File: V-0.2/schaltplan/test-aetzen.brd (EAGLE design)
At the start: 78.6 x 50.8 mm, 53 parts, among them IC1 MEGA32-A, IC2 NE5532N, Q1 BUZ21, X1 BU-SMB-H, X2 PN61729-S

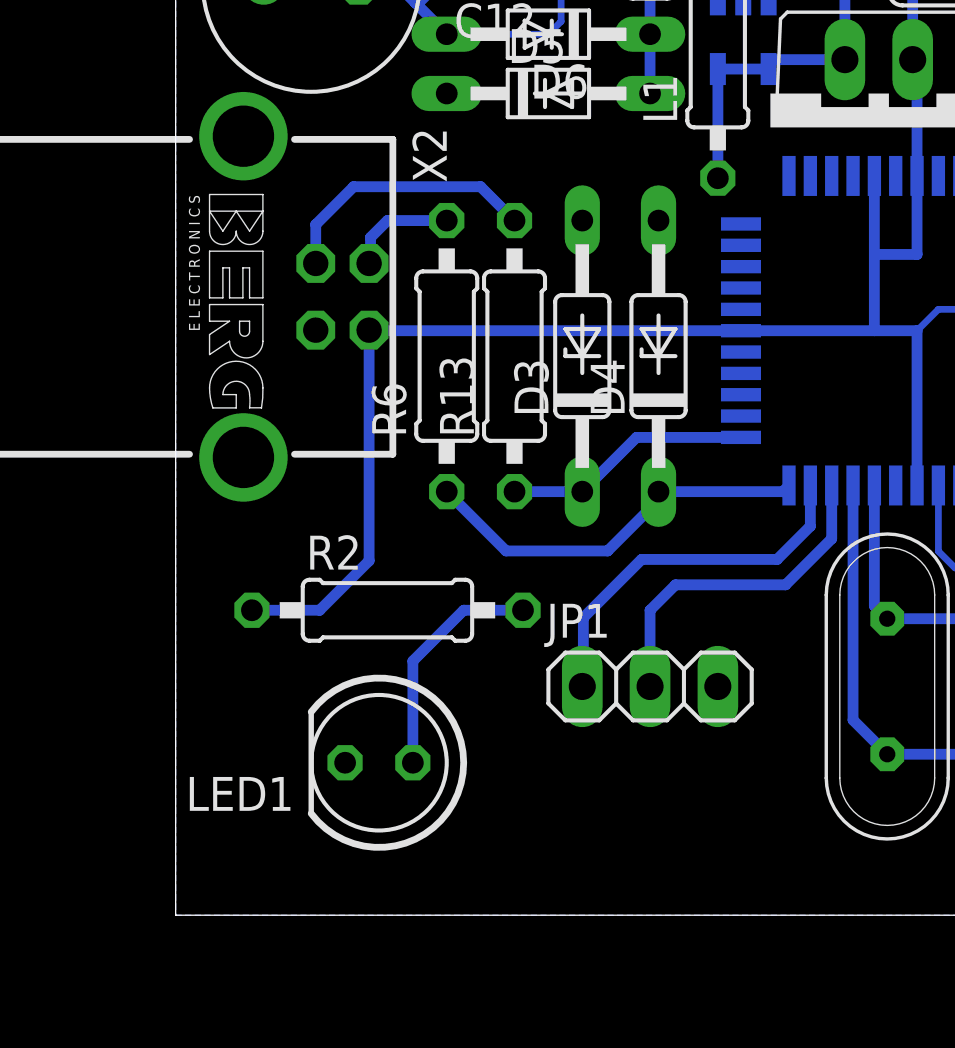
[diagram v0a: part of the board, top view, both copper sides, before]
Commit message: i have no flash drive with me :(
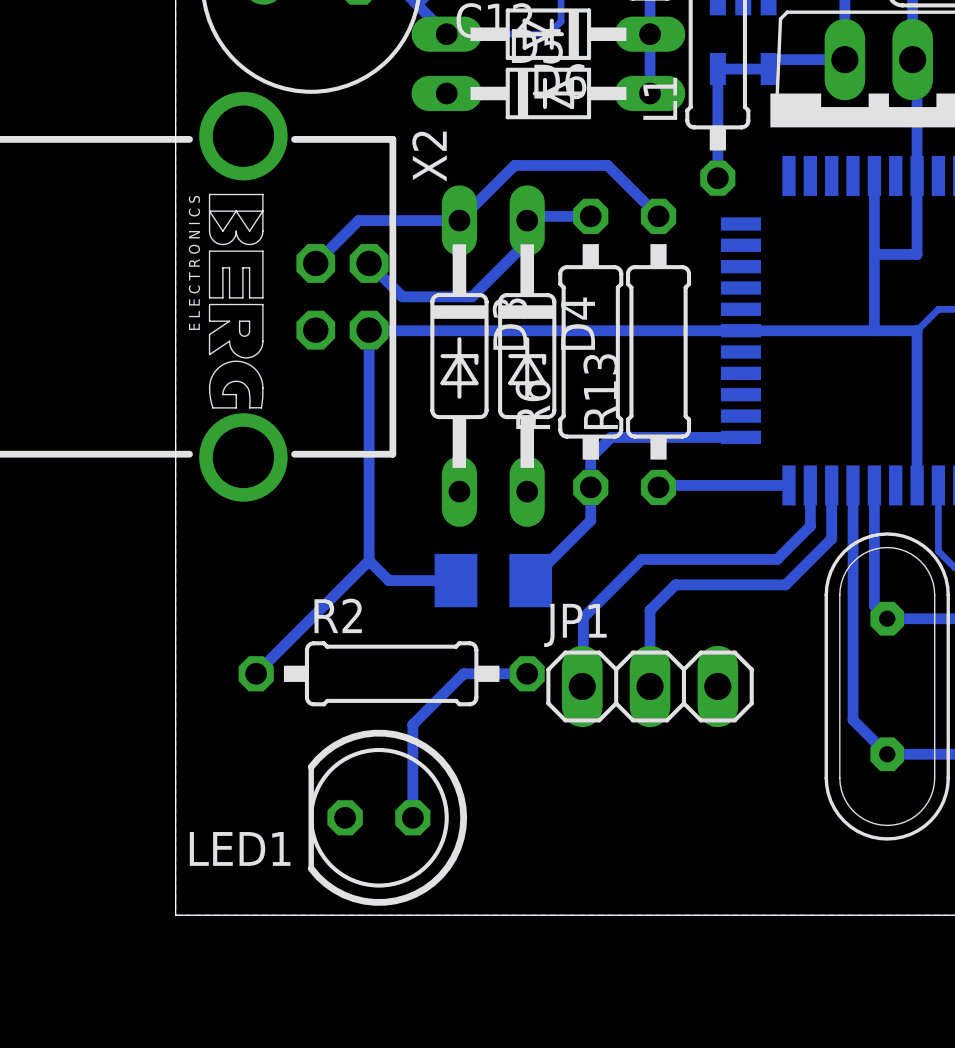
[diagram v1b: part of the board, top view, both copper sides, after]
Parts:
- added R17: 10k, rcl:M1206
- moved R13 5.40 mm to (18.1, 21.1)
- moved R6 5.40 mm to (15.6, 21.1)
- moved D4 4.92 mm to (13.2, 21.0), turned to 270 degrees
- moved D3 4.60 mm to (10.6, 21.0), turned to 270 degrees
- moved R2 2.39 mm to (8.10, 9.05)
- moved LED1 2.06 mm to (7.62, 3.65)
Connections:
- net N$13: now also D4.C
- net N$14: now also D3.C
- net N$2: now also IC1.12, R17.2; no longer D4.C, IC1.11
- net N$5: now also IC1.11; no longer D3.C, IC1.12
- net VCC: now also R17.1
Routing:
- net N$13: track 4.11 -> 10.5 mm
- net N$14: track 10.0 -> 15.2 mm
- net N$5: track 9.33 -> 4.92 mm
- net VCC: track 124.4 -> 128.8 mm
- net N$2: track 15.0 -> 11.5 mm
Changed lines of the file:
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@@
 <layer number="22" name="bPlace" color="7" fill="1" visible="no" active="yes"/>
 <layer number="23" name="tOrigins" color="15" fill="1" visible="yes" active="yes"/>
-<layer number="24" name="bOrigins" color="15" fill="1" visible="no" active="yes"/>
+<layer number="24" name="bOrigins" color="15" fill="1" visible="yes" active="yes"/>
 <layer number="25" name="tNames" color="7" fill="1" visible="yes" active="yes"/>
 <layer number="26" name="bNames" color="7" fill="1" visible="no" active="yes"/>
@@
 <element name="D1" library="diode" package="DO35-7" value="1N4148DO35-7" x="44.45" y="37.465"/>
 <element name="D2" library="diode" package="DO35-7" value="1N4148DO35-7" x="44.45" y="35.2425" rot="R180"/>
-<element name="D3" library="diode" package="DO35Z10" value="" x="15.24" y="20.955" rot="R90"/>
-<element name="D4" library="diode" package="DO35Z10" value="" x="18.0975" y="20.955" rot="R90"/>
+<element name="D3" library="diode" package="DO35Z10" value="" x="10.63625" y="20.955" rot="R270"/>
+<element name="D4" library="diode" package="DO35Z10" value="" x="13.17625" y="20.955" rot="R270"/>
 <element name="D5" library="diode" package="DO34-7" value="BAT81" x="13.97" y="30.7975"/>
 <element name="D6" library="diode" package="DO34-7" value="BAT81" x="13.97" y="33.02" rot="R180"/>
@@
 <element name="JP2" library="jumper" package="JP4Q" value="" x="54.13375" y="27.78125" rot="R90"/>
 <element name="L1" library="rcl" package="0207/10" value="" x="20.32" y="32.7025" rot="R90"/>
-<element name="LED1" library="led" package="LED5MM" value="" x="7.62" y="5.715" rot="R180"/>
+<element name="LED1" library="led" package="LED5MM" value="" x="7.62" y="3.65125" rot="R180"/>
 <element name="Q1" library="transistor-fet" package="TO220V" value="BUZ21" x="27.6225" y="29.5275" rot="R180"/>
 <element name="QG1" library="crystal" package="SM77H" value="SM77H" x="43.18" y="15.24" rot="MR0">
@@
 <element name="R11" library="rcl" package="M1206" value="10k" x="63.02375" y="16.98625" rot="MR0"/>
 <element name="R12" library="rcl" package="M1206" value="10k" x="59.84875" y="9.2075" rot="MR270"/>
-<element name="R13" library="rcl" package="0207/10" value="33R" x="12.7" y="20.955" rot="R90"/>
-<element name="R2" library="rcl" package="0207/10" value="" x="7.9375" y="11.43"/>
+<element name="R13" library="rcl" package="0207/10" value="33R" x="18.0975" y="21.11375" rot="R90"/>
+<element name="R2" library="rcl" package="0207/10" value="" x="8.09625" y="9.04875"/>
 <element name="R3" library="rcl" package="RTRIM64Y" value="" x="70.32625" y="23.65375" rot="R270"/>
 <element name="R4" library="rcl" package="M1206" value="10k" x="34.925" y="6.0325" rot="MR270"/>
 <element name="R5" library="rcl" package="M1206" value="10k" x="34.6075" y="29.5275" rot="MR0"/>
-<element name="R6" library="rcl" package="0207/10" value="33R" x="10.16" y="20.955" rot="R90"/>
+<element name="R6" library="rcl" package="0207/10" value="33R" x="15.5575" y="21.11375" rot="R90"/>
 <element name="R7" library="rcl" package="0207/10" value="" x="17.145" y="40.64" rot="R180"/>
 <element name="R8" library="rcl" package="0207/10" value="" x="17.145" y="43.18"/>
@@
 <element name="JP1" library="pinhead" package="1X03" value="" x="17.78" y="8.5725"/>
 <element name="R16" library="rcl" package="M1206" value="10k" x="33.17875" y="37.30625" rot="MR270"/>
+<element name="R17" library="rcl" package="M1206" value="10k" x="11.90625" y="12.54125" rot="MR180"/>
 </elements>
 <signals>
@@
 <contactref element="R4" pad="2"/>
 <wire x1="7.25" y1="21.9275" x2="7.25" y2="13.2825" width="0.4064" layer="16"/>
-<wire x1="7.25" y1="13.2825" x2="5.3975" y2="11.43" width="0.4064" layer="16"/>
-<wire x1="5.3975" y1="11.43" x2="2.8575" y2="11.43" width="0.4064" layer="16"/>
+<wire x1="7.25" y1="13.2825" x2="3.01625" y2="9.04875" width="0.4064" layer="16"/>
 <wire x1="45.085" y1="5.08" x2="45.085" y2="3.175" width="0.4064" layer="16"/>
 <wire x1="45.085" y1="3.175" x2="44.1325" y2="2.2225" width="0.4064" layer="16"/>
@@
 <wire x1="28.41625" y1="37.30625" x2="27.6225" y2="36.5125" width="0.254" layer="16"/>
 <wire x1="27.6225" y1="36.5125" x2="27.6225" y2="35.2425" width="0.254" layer="16"/>
+<contactref element="R17" pad="1"/>
+<wire x1="10.50625" y1="12.54125" x2="7.99125" y2="12.54125" width="0.4064" layer="16"/>
+<wire x1="7.99125" y1="12.54125" x2="7.25" y2="13.2825" width="0.4064" layer="16"/>
 <wire x1="45.73" y1="13.34" x2="45.085" y2="5.08" width="0" layer="19" extent="16-16"/>
 </signal>
@@
 <contactref element="R2" pad="2"/>
 <contactref element="LED1" pad="A"/>
-<wire x1="13.0175" y1="11.43" x2="10.795" y2="11.43" width="0.4064" layer="16"/>
-<wire x1="10.795" y1="11.43" x2="8.89" y2="9.525" width="0.4064" layer="16"/>
-<wire x1="8.89" y1="9.525" x2="8.89" y2="5.715" width="0.4064" layer="16"/>
+<wire x1="13.17625" y1="9.04875" x2="10.795" y2="9.04875" width="0.4064" layer="16"/>
+<wire x1="10.795" y1="9.04875" x2="8.89" y2="7.14375" width="0.4064" layer="16"/>
+<wire x1="8.89" y1="7.14375" x2="8.89" y2="3.65125" width="0.4064" layer="16"/>
 </signal>
 <signal name="N$25">
@@
 </signal>
 <signal name="N$2">
+<contactref element="R6" pad="1"/>
+<contactref element="IC1" pad="12"/>
+<contactref element="R17" pad="2"/>
+<wire x1="21.1875" y1="17.9075" x2="16.32" y2="17.9075" width="0.4064" layer="16"/>
+<wire x1="16.32" y1="17.9075" x2="15.5575" y2="17.145" width="0.4064" layer="16"/>
+<wire x1="15.5575" y1="17.145" x2="15.5575" y2="16.03375" width="0.4064" layer="16"/>
+<wire x1="15.5575" y1="16.03375" x2="15.5575" y2="14.7925" width="0.4064" layer="16"/>
+<wire x1="15.5575" y1="14.7925" x2="13.30625" y2="12.54125" width="0.4064" layer="16"/>
+</signal>
+<signal name="N$5">
+<contactref element="R13" pad="1"/>
 <contactref element="IC1" pad="11"/>
-<contactref element="R6" pad="1"/>
-<contactref element="D4" pad="C"/>
-<wire x1="10.16" y1="15.875" x2="12.3825" y2="13.6525" width="0.4064" layer="16"/>
-<wire x1="12.3825" y1="13.6525" x2="16.1925" y2="13.6525" width="0.4064" layer="16"/>
-<wire x1="16.1925" y1="13.6525" x2="18.0975" y2="15.5575" width="0.4064" layer="16"/>
-<wire x1="18.0975" y1="15.5575" x2="18.0975" y2="15.875" width="0.4064" layer="16"/>
-<wire x1="22.9875" y1="16.1075" x2="22.755" y2="15.875" width="0.4064" layer="16"/>
-<wire x1="22.755" y1="15.875" x2="18.0975" y2="15.875" width="0.4064" layer="16"/>
-</signal>
-<signal name="N$5">
-<contactref element="IC1" pad="12"/>
-<contactref element="R13" pad="1"/>
-<contactref element="D3" pad="C"/>
-<wire x1="12.7" y1="15.875" x2="15.24" y2="15.875" width="0.4064" layer="16"/>
-<wire x1="15.24" y1="15.875" x2="17.2725" y2="17.9075" width="0.4064" layer="16"/>
-<wire x1="17.2725" y1="17.9075" x2="21.1875" y2="17.9075" width="0.4064" layer="16"/>
+<wire x1="22.9875" y1="16.1075" x2="18.17125" y2="16.1075" width="0.4064" layer="16"/>
+<wire x1="18.17125" y1="16.1075" x2="18.0975" y2="16.03375" width="0.4064" layer="16"/>
 </signal>
 <signal name="N$1">
@@
 <contactref element="X2" pad="2"/>
 <contactref element="R6" pad="2"/>
-<wire x1="10.16" y1="26.035" x2="7.9375" y2="26.035" width="0.4064" layer="16"/>
-<wire x1="7.9375" y1="26.035" x2="7.3025" y2="25.4" width="0.4064" layer="16"/>
-<wire x1="7.3025" y1="25.4" x2="7.3025" y2="24.48" width="0.4064" layer="16"/>
-<wire x1="7.3025" y1="24.48" x2="7.25" y2="24.4275" width="0.4064" layer="16"/>
+<contactref element="D4" pad="C"/>
+<wire x1="7.25" y1="24.4275" x2="8.5" y2="23.1775" width="0.4064" layer="16"/>
+<wire x1="8.5" y1="23.1775" x2="11.1125" y2="23.1775" width="0.4064" layer="16"/>
+<wire x1="11.1125" y1="23.1775" x2="13.17625" y2="25.24125" width="0.4064" layer="16"/>
+<wire x1="13.17625" y1="25.24125" x2="13.17625" y2="26.035" width="0.4064" layer="16"/>
+<wire x1="13.17625" y1="26.035" x2="13.335" y2="26.19375" width="0.4064" layer="16"/>
+<wire x1="13.335" y1="26.19375" x2="15.5575" y2="26.19375" width="0.4064" layer="16"/>
 </signal>
 <signal name="N$14">
 <contactref element="X2" pad="3"/>
 <contactref element="R13" pad="2"/>
-<wire x1="12.7" y1="26.035" x2="11.43" y2="27.305" width="0.4064" layer="16"/>
-<wire x1="11.43" y1="27.305" x2="6.6675" y2="27.305" width="0.4064" layer="16"/>
-<wire x1="6.6675" y1="27.305" x2="5.25" y2="25.8875" width="0.4064" layer="16"/>
-<wire x1="5.25" y1="25.8875" x2="5.25" y2="24.4275" width="0.4064" layer="16"/>
+<contactref element="D3" pad="C"/>
+<wire x1="5.25" y1="24.4275" x2="6.8575" y2="26.035" width="0.4064" layer="16"/>
+<wire x1="6.8575" y1="26.035" x2="10.63625" y2="26.035" width="0.4064" layer="16"/>
+<wire x1="10.63625" y1="26.035" x2="12.7" y2="28.09875" width="0.4064" layer="16"/>
+<wire x1="12.7" y1="28.09875" x2="16.1925" y2="28.09875" width="0.4064" layer="16"/>
+<wire x1="16.1925" y1="28.09875" x2="18.0975" y2="26.19375" width="0.4064" layer="16"/>
 </signal>
 <signal name="N$15">
